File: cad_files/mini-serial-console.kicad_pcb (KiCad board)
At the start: 2 copper layers, 97.8 x 59.7 mm, 49 parts, among them J1 Screw_Terminal_1x02, J2 Screw_Terminal_1x03, J3 Screw_Terminal_1x03, J4 Screw_Terminal_1x07, Q1 BC559, Q2 BC548, Q3 BC109, U1 HD44780 compatible LCD, U2 Raspberry Pi Pico

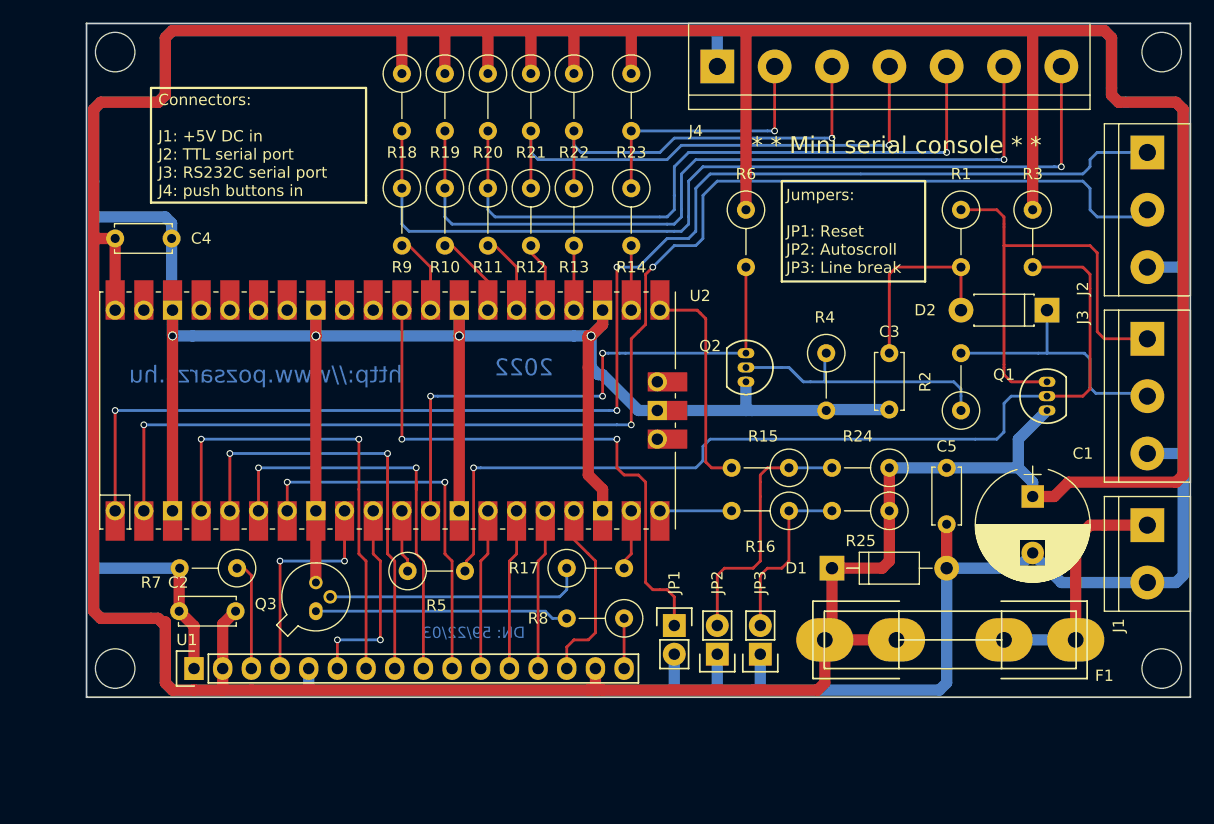
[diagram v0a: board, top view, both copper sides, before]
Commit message: 221018
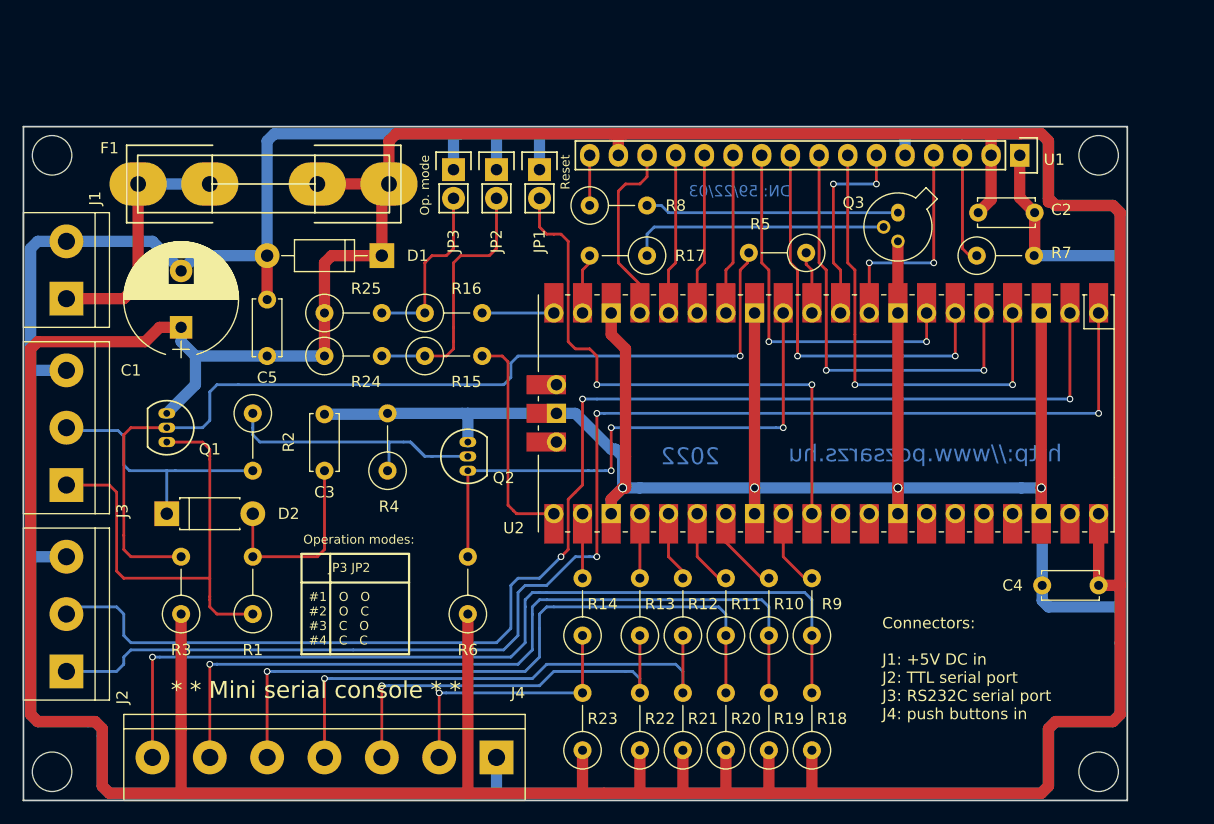
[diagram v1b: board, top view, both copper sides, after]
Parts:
- moved REF** 117.2 mm to (98.6, 126.0), turned to 180 degrees
- moved REF** 108.3 mm to (98.6, 71.4), turned to 180 degrees
- moved REF** 108.0 mm to (191.3, 126.0), turned to 180 degrees
- moved J2 106.2 mm to (99.8, 117.1), turned to 90 degrees
- moved REF** 98.3 mm to (191.3, 71.4), turned to 180 degrees
- moved J1 97.8 mm to (99.8, 84.1), turned to 90 degrees
- moved J3 96.6 mm to (99.8, 100.6), turned to 90 degrees
- moved C4 92.4 mm to (191.3, 109.5), turned to 180 degrees
- moved U1 86.1 mm to (184.3, 71.4), turned to 180 degrees
- moved R3 83.5 mm to (110.0, 112.0), turned to 90 degrees
- moved D2 80.0 mm to (108.7, 103.1), turned to 0 degrees
- moved Q1 78.0 mm to (108.7, 94.2), turned to 270 degrees
- moved C1 76.9 mm to (110.0, 86.6), turned to 90 degrees
- moved C2 74.7 mm to (180.6, 76.5), turned to 0 degrees
- moved F1 72.5 mm to (117.6, 73.9), turned to 180 degrees
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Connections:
- JP1 pad 1: Net-(JP1-Pad1) -> GND
- JP1 pad 2: GND -> Net-(JP1-Pad2)
- U2 pad 30: Net-(JP1-Pad1) -> Net-(JP1-Pad2)
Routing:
- net Net-(JP1-Pad1): track 50.6 -> 0.00 mm, vias 2 -> 0
- net Net-(JP1-Pad2): track 0.00 -> 50.6 mm, vias 0 -> 2
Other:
- board text added: "JP3 JP2 #1 O O #2 O C #3 C O #4 C C"
- board text added: "Op. mode"
- board text added: "Operation modes:"
- board text added: "Reset"
- board text removed: "Jumpers: JP1: Reset JP2: Autoscroll JP3: Line break"
